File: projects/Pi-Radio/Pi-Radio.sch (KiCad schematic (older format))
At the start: 23 parts, among them J1 Data, J8 Power, SW1 Left, SW2 Time, SW3 Up, SW4 JazMan, SW5 PlayStop, SW6 Down, SW7 Right

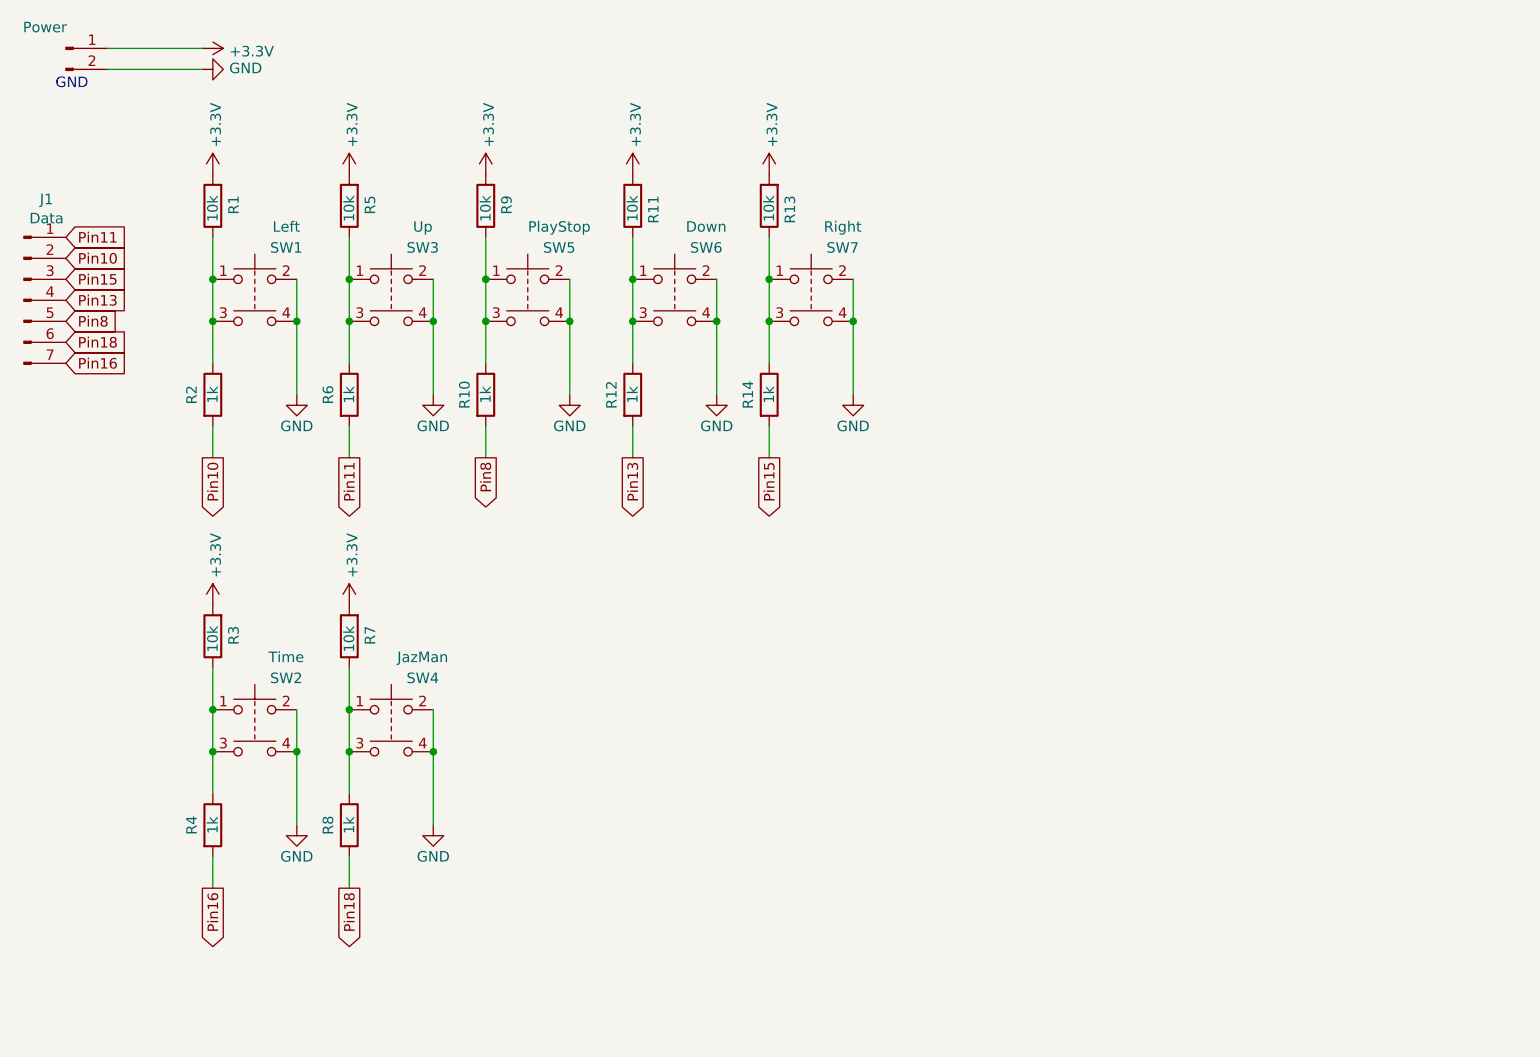
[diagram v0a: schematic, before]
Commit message: updates
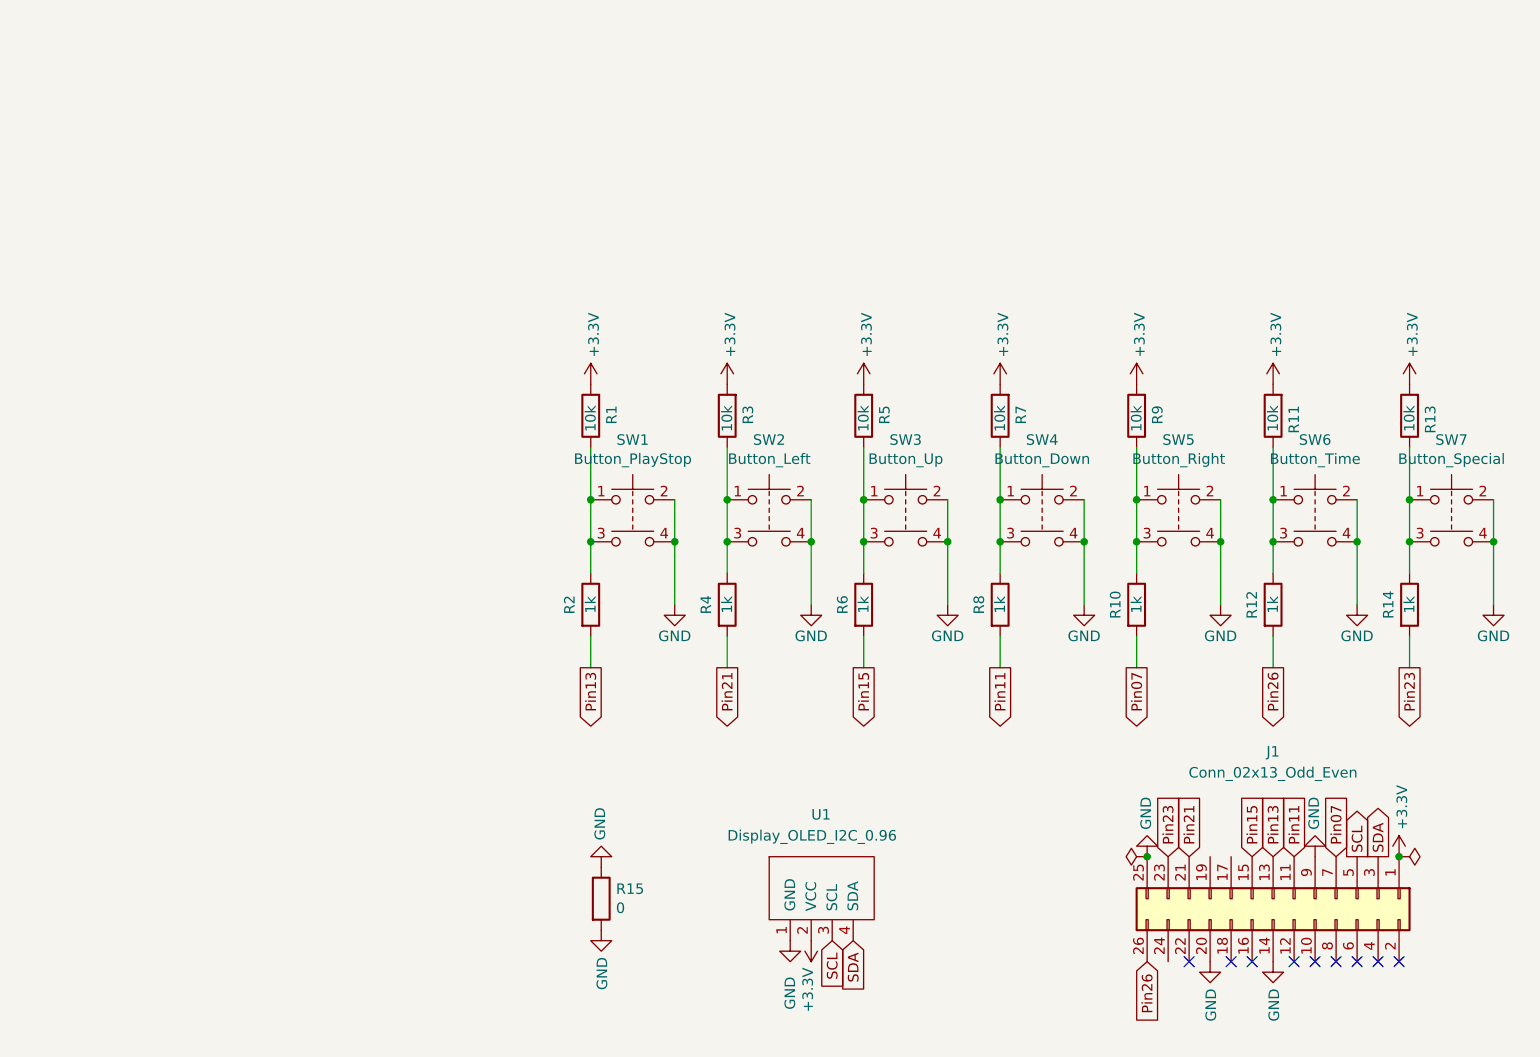
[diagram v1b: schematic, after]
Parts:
- removed J1: Data, Connector_PinHeader_2.54mm:PinHeader_1x07_P2.54mm_Vertical, symbol Connector:Conn_01x07_Male
- removed J8: Power, Connector_PinHeader_2.54mm:PinHeader_1x02_P2.54mm_Vertical, symbol Connector:Conn_01x02_Male
- added J1: Conn_02x13_Odd_Even, Connector_PinSocket_2.54mm:PinSocket_2x13_P2.54mm_Vertical, symbol Connector_Generic:Conn_02x13_Odd_Even
- added R15: 0, Resistor_THT:R_Axial_DIN0204_L3.6mm_D1.6mm_P7.62mm_Horizontal, symbol Device:R
- added U1: Display_OLED_I2C_0.96, OLED:Display_128x64_096_I2C, symbol OLED:Display_OLED_I2C_0.96
- SW1: value Left -> Button_PlayStop; footprint Button_Switch_THT:SW_PUSH_6mm_H5mm -> Button_Switch_THT:SW_PUSH_6mm
- SW2: value Time -> Button_Left; footprint Button_Switch_THT:SW_PUSH_6mm_H5mm -> Button_Switch_THT:SW_PUSH_6mm
- SW3: value Up -> Button_Up; footprint Button_Switch_THT:SW_PUSH_6mm_H5mm -> Button_Switch_THT:SW_PUSH_6mm
- SW4: value JazMan -> Button_Down; footprint Button_Switch_THT:SW_PUSH_6mm_H5mm -> Button_Switch_THT:SW_PUSH_6mm
- SW5: value PlayStop -> Button_Right; footprint Button_Switch_THT:SW_PUSH_6mm_H5mm -> Button_Switch_THT:SW_PUSH_6mm
- SW6: value Down -> Button_Time; footprint Button_Switch_THT:SW_PUSH_6mm_H5mm -> Button_Switch_THT:SW_PUSH_6mm
- SW7: value Right -> Button_Special; footprint Button_Switch_THT:SW_PUSH_6mm_H5mm -> Button_Switch_THT:SW_PUSH_6mm
- renumbered R9 to R1, R14 to R10, R3 to R11, R4 to R12, R7 to R13, R8 to R14, R10 to R2, R1 to R3, R2 to R4, R11 to R7, R12 to R8, R13 to R9
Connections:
- net Pin8 is gone; now on net Pin13: R2.2
- net +3V3: now also J1.1 (Pin_1), U1.2 (VCC)
- net GND: now also J1.14 (Pin_14), J1.20 (Pin_20), J1.25 (Pin_25), J1.9 (Pin_9), R15.1, R15.2, U1.1 (GND)
- net Pin11: now also R8.2, J1.11 (Pin_11); no longer R6.2
- net Pin13: now also J1.13 (Pin_13); no longer R8.2
- net Pin15: now also R6.2, J1.15 (Pin_15); no longer R10.2
- net at R3.1, R4.1: now also SW2.1, SW2.3; no longer SW1.1, SW1.3
- net at R1.1, R2.1: now also SW1.1, SW1.3; no longer SW5.1, SW5.3
- net at R7.1, R8.1: now also SW4.1, SW4.3; no longer SW6.1, SW6.3
- net at R10.1, R9.1: now also SW5.1, SW5.3; no longer SW7.1, SW7.3
- net at R11.1, R12.1: now also SW6.1, SW6.3; no longer SW2.1, SW2.3
- net at R13.1, R14.1: now also SW7.1, SW7.3; no longer SW4.1, SW4.3
- net Pin10 renamed Pin21
- net Pin21: now also J1.21 (Pin_21)
- net Pin16 renamed Pin26
- net Pin26: now also J1.26 (Pin_26)
- net Pin18 renamed Pin23
- net Pin23: now also J1.23 (Pin_23)
- new net Pin07: J1.7 (Pin_7), R10.2
- new net SCL: J1.5 (Pin_5), U1.3 (SCL)
- new net SDA: J1.3 (Pin_3), U1.4 (SDA)
- no-connect marks 0 -> 9
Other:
- note removed: "GND"
- moved on the sheet: R1, R10, R11, R12, R13, R14, R2, R3, R4, R5, R6, R7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
